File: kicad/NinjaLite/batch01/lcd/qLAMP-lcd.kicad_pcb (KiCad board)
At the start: 2 copper layers, 39 x 28.5 mm, 22 parts, among them J1 Conn_01x04_Male, J2 Conn_01x04_Male, J3 Conn_01x04_Male, Q1 Q_NPN_BEC, Q2 Q_NPN_BEC, Q3 Q_NPN_BEC, SW1 TACTILE_4, SW2 TACTILE_4, SW3 TACTILE_4

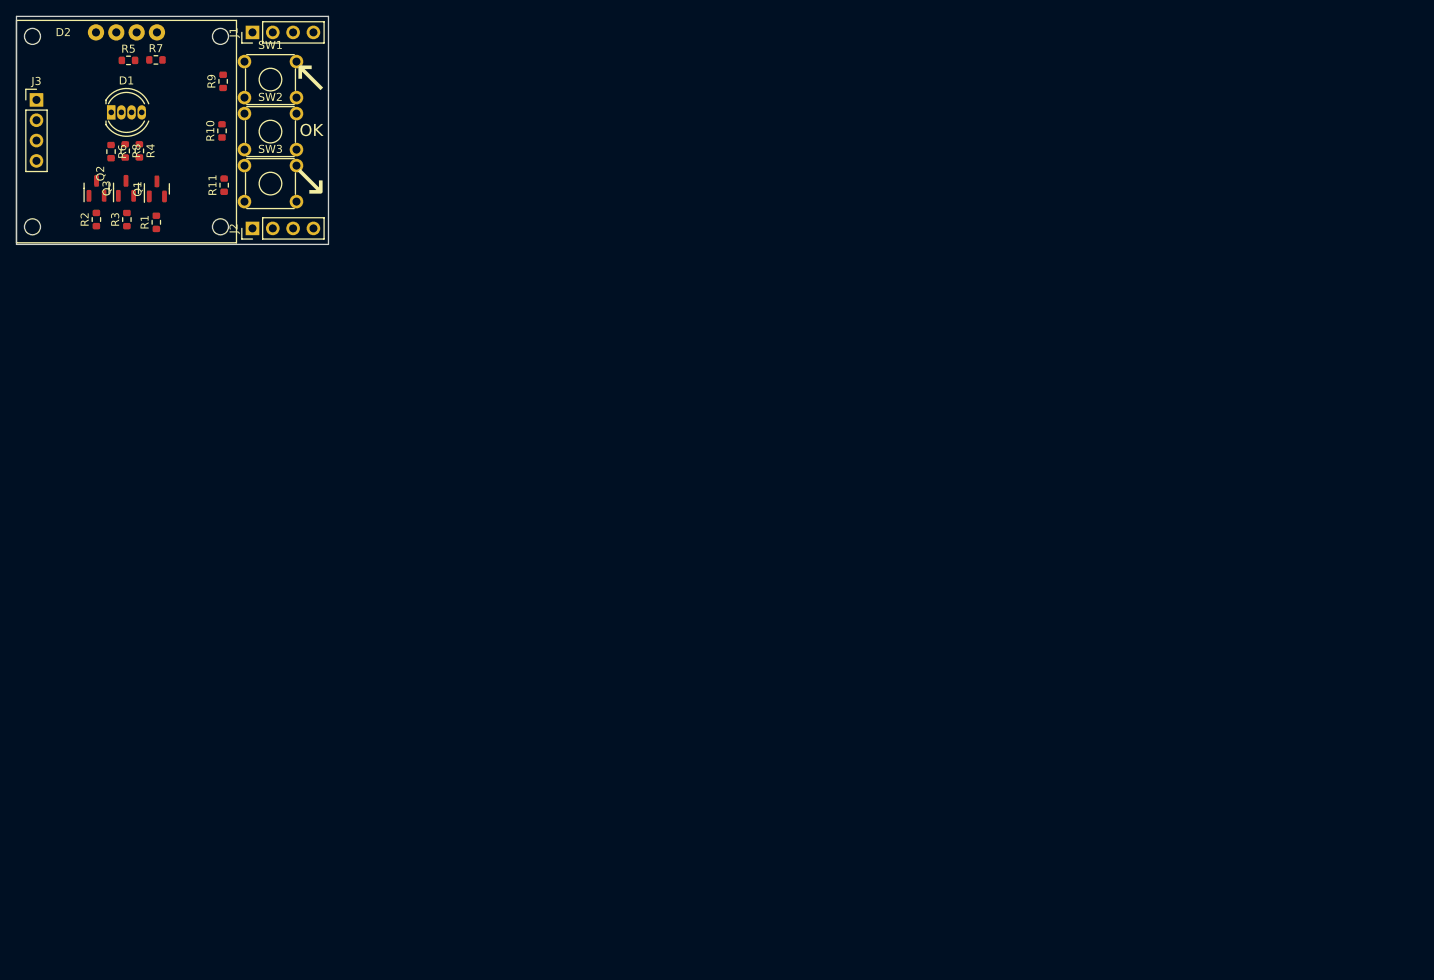
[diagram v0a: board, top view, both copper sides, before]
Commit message: batch01 ready
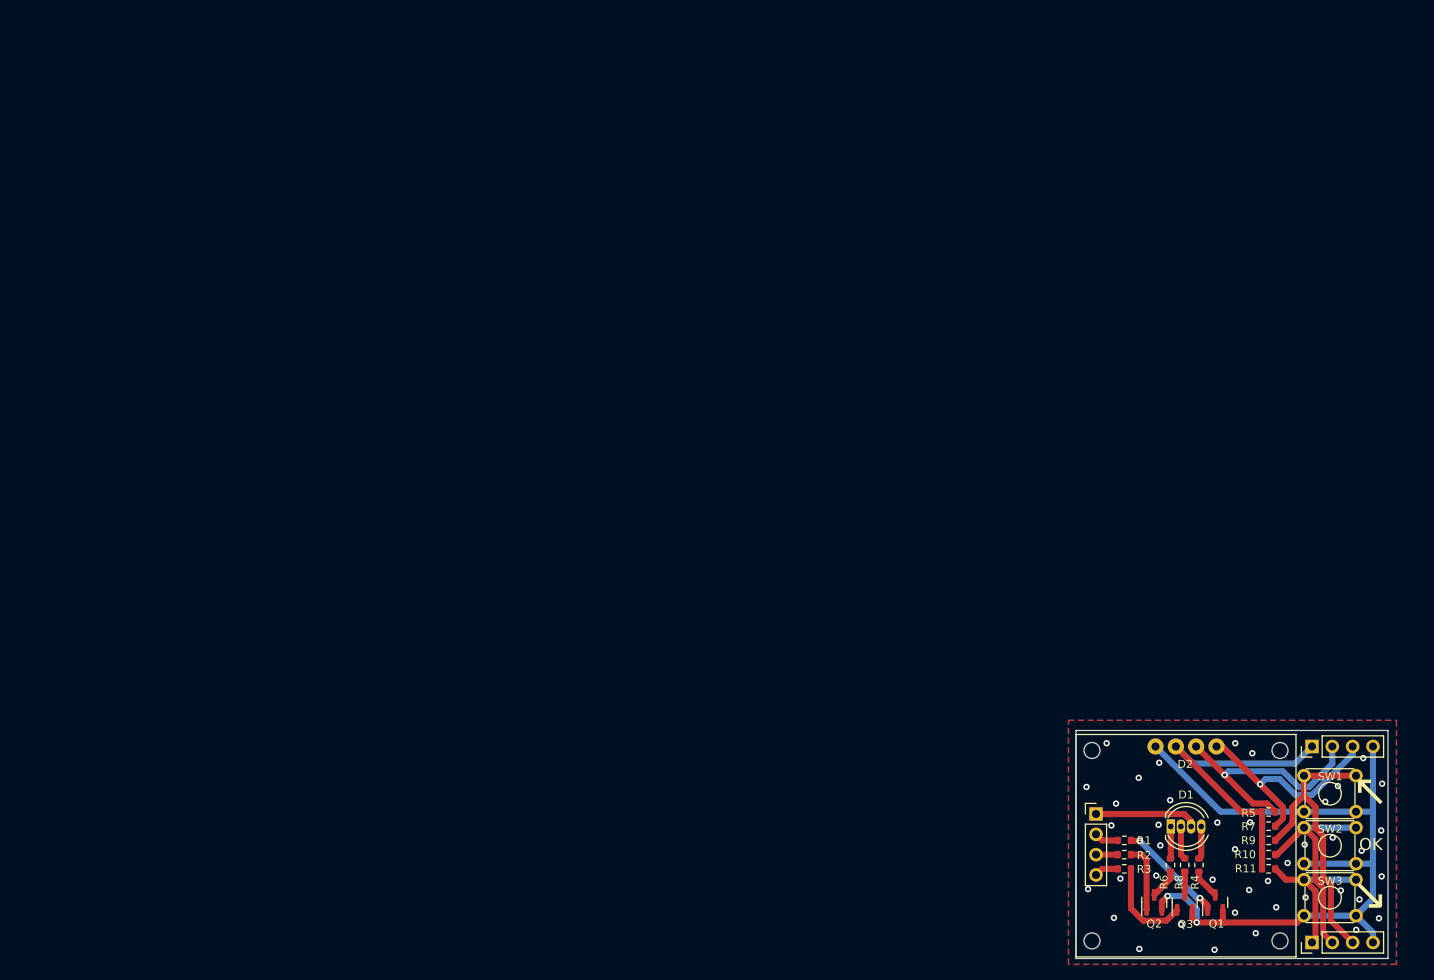
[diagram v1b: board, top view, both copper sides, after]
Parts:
- moved R5 170.7 mm to (156.5, 99.4)
- moved R7 168.9 mm to (156.5, 101.2)
- moved R9 161.5 mm to (156.5, 103.0), turned to 0 degrees
- moved R4 159.7 mm to (147.8, 106.1)
- moved D1 159.7 mm to (144.3, 101.3)
- moved D2 159.7 mm to (146.2, 89.8)
- moved J1 159.7 mm to (161.9, 91.3)
- moved J2 159.7 mm to (161.9, 115.8)
- moved J3 159.7 mm to (134.9, 99.7)
- moved SW1 159.7 mm to (160.9, 94.9)
- moved SW2 159.7 mm to (160.9, 101.4)
- moved SW3 159.7 mm to (160.9, 107.9)
- moved R8 159.7 mm to (146.0, 106.1)
- moved R6 159.7 mm to (144.3, 106.1)
- moved Q3 159.6 mm to (146.0, 110.8)
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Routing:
- net GND: track 0.00 -> 97.3 mm, vias 0 -> 44
- net VCC: track 0.00 -> 40.1 mm
- net TACT1: track 0.00 -> 37.0 mm
- net SCL: track 0.00 -> 31.1 mm, vias 0 -> 1
- net SDA: track 0.00 -> 30.0 mm, vias 0 -> 1
- net TACT2: track 0.00 -> 27.3 mm
- net TACT3: track 0.00 -> 19.3 mm
- net Net-(Q1-Pad1): track 0.00 -> 13.5 mm, vias 0 -> 2
- net VCCL: track 0.00 -> 12.9 mm
- net Net-(Q3-Pad1): track 0.00 -> 11.9 mm
- net Net-(Q2-Pad1): track 0.00 -> 8.50 mm
- net Net-(D1-Pad2): track 0.00 -> 4.19 mm
- net Net-(D1-Pad4): track 0.00 -> 4.11 mm
- net Net-(D1-Pad1): track 0.00 -> 4.01 mm
- net Net-(Q2-Pad3): track 0.00 -> 3.75 mm
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- added copper zone on B.Cu, net GND
- added copper zone on F.Cu, net GND

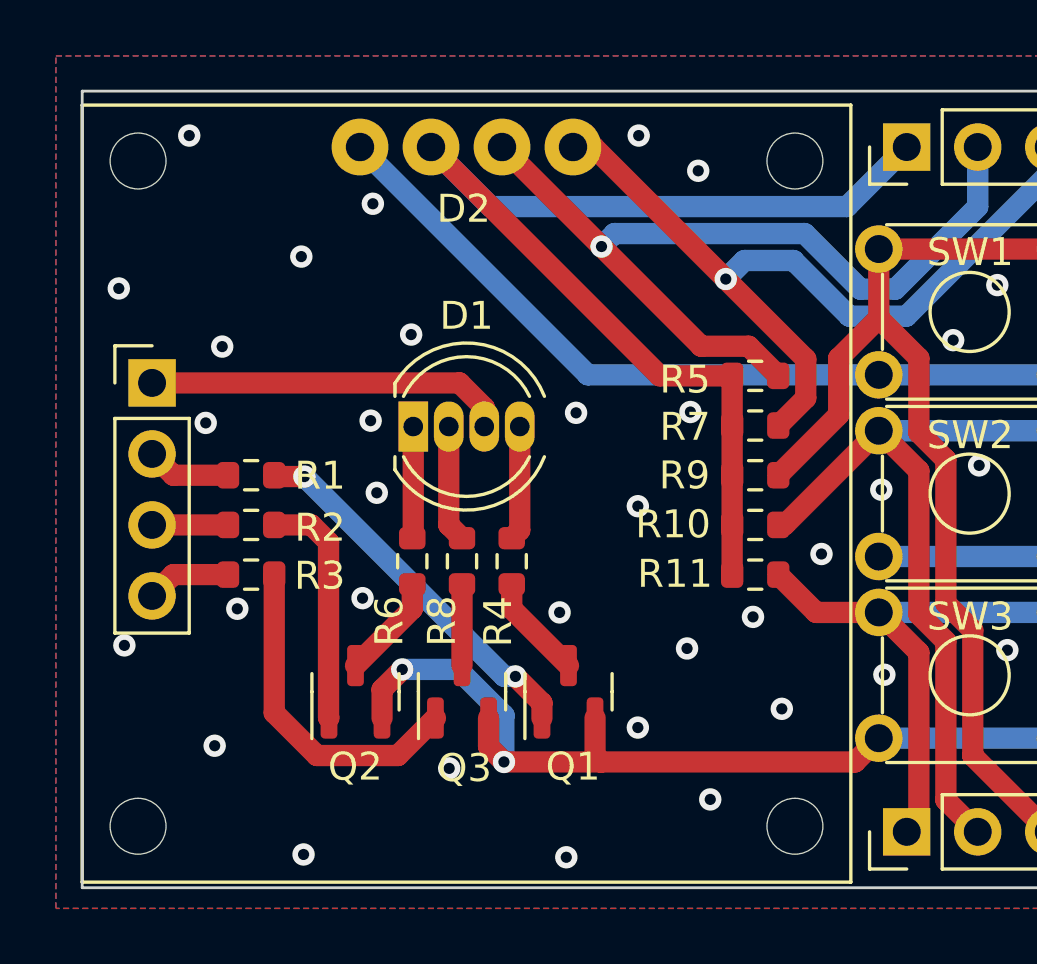
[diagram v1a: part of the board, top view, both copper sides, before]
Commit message: batch01 ready
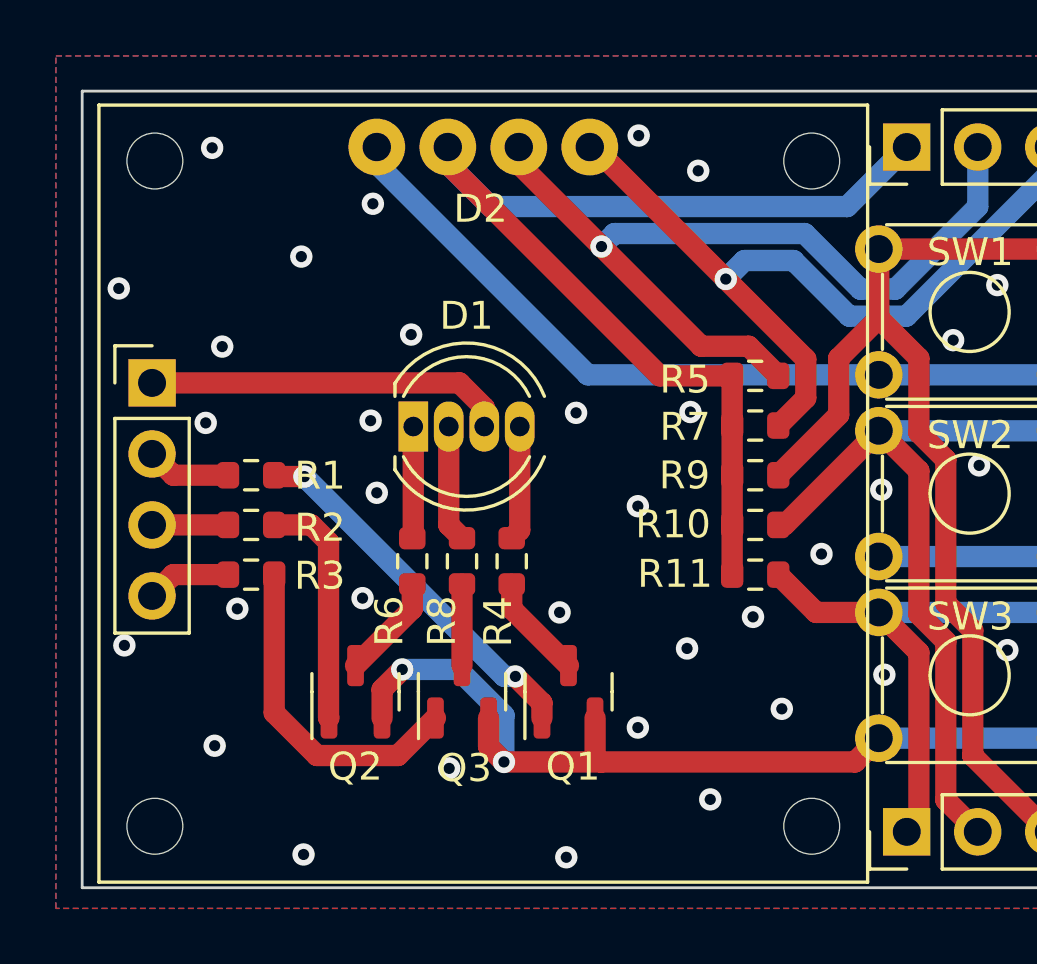
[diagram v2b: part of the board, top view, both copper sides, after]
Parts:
- moved D2 0.60 mm to (146.8, 89.8)
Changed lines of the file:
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@@
   (net 20 "VCCL")
   (footprint "Ninja-qPCR:I2C_SSD1306_LCD" (layer "F.Cu")
-    (at 146.19 89.76)
+    (at 146.790004 89.759993)
     (property "Sheetfile" "qLAMP-lcd.kicad_sch")
     (property "Sheetname" "")
@@
     (pad "4" thru_hole oval locked (at 3.81 1.5) (size 2.032 2.032) (drill 1.016) (layers *.Cu *.Mask)
       (net 13 "SDA") (pinfunction "SDA") (pintype "input"))
-    (model ":desktop:I2C_SSD1306_LCD v1.step"
+    (model ":desktop:I2C_SSD1306_LCD v1.step" hide
       (offset (xyz 0 0 0))
       (scale (xyz 1 1 1))
@@
   (segment (start 147.53 113.26) (end 146.979 112.709) (width 0.762) (layer "F.Cu") (net 19))
   (via (at 142.84 93.29) (size 0.8) (drill 0.4) (layers "F.Cu" "B.Cu") (free) (net 19))
-  (via (at 136.27 90.85) (size 0.8) (drill 0.4) (layers "F.Cu" "B.Cu") (free) (net 19))
+  (via (at 137.09 91.29) (size 0.8) (drill 0.4) (layers "F.Cu" "B.Cu") (free) (net 19))
   (via (at 152.32 104.11) (size 0.8) (drill 0.4) (layers "F.Cu" "B.Cu") (free) (net 19))
   (via (at 150.11 100.77) (size 0.8) (drill 0.4) (layers "F.Cu" "B.Cu") (free) (net 19))
